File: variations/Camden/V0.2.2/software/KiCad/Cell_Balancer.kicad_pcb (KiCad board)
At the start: 2 copper layers, 14 parts, among them J1 Screw_Terminal_01x11, J2 DC37_Pins

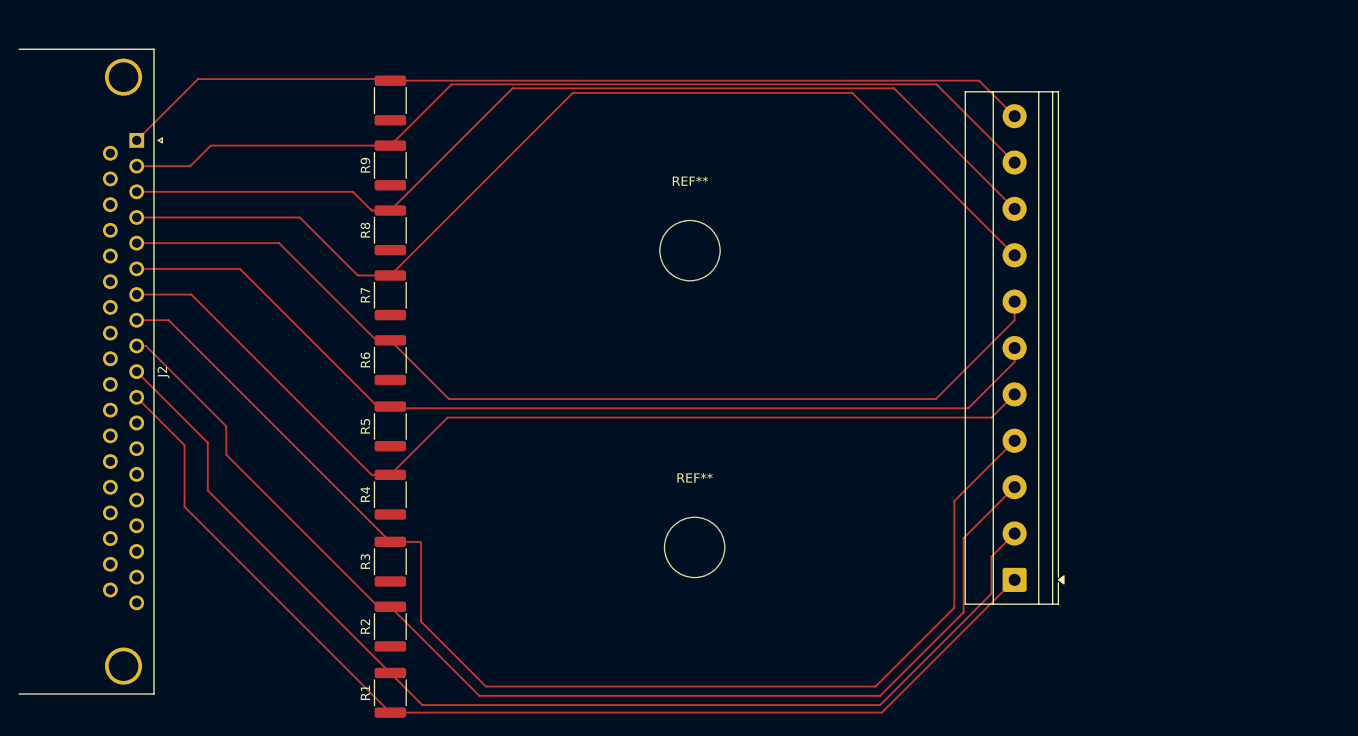
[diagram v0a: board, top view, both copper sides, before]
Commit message: update
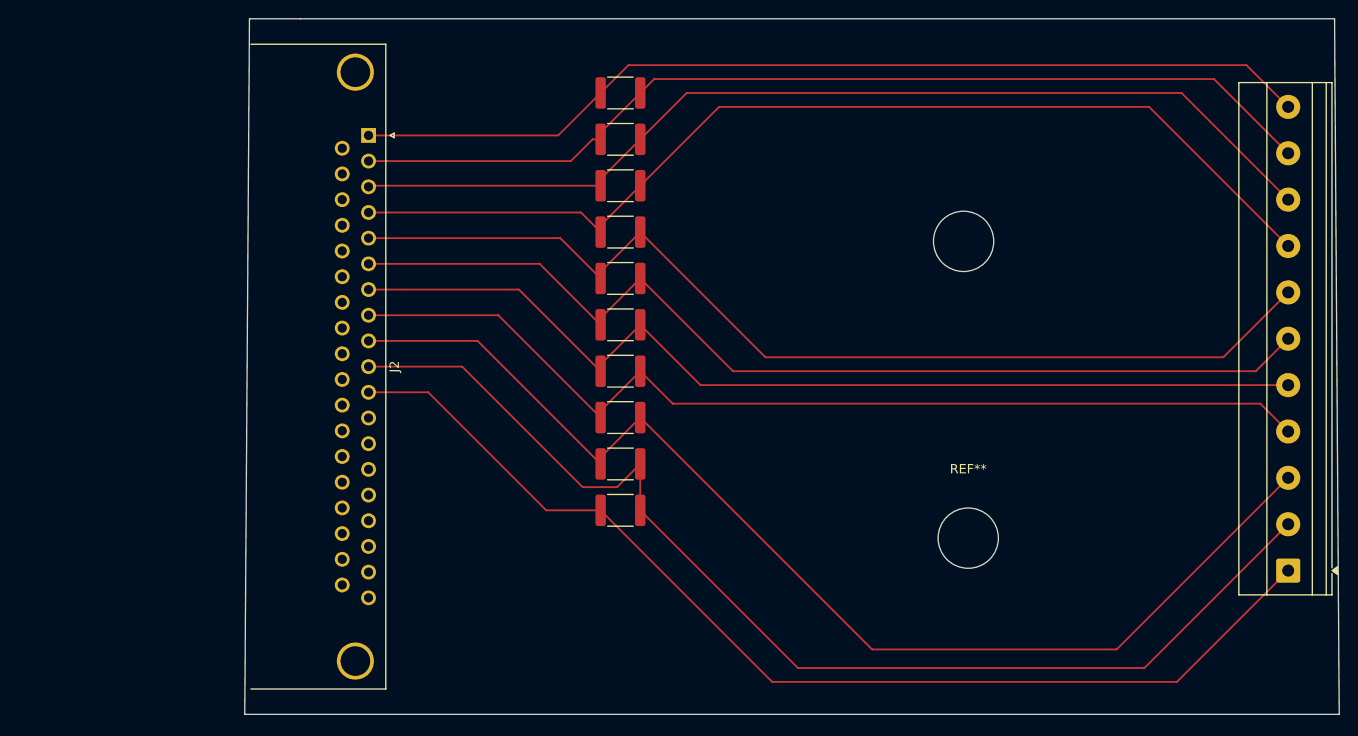
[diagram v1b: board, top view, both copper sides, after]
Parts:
- moved R1 31.7 mm to (124.5, 128.0), turned to 0 degrees
- moved R2 30.4 mm to (124.5, 123.0), turned to 180 degrees
- moved J1 29.5 mm to (196.5, 134.5)
- moved REF** 29.5 mm to (161.5, 99.0)
- moved REF** 29.5 mm to (162.0, 131.0)
- moved R3 29.3 mm to (124.5, 118.0), turned to 180 degrees
- moved R4 28.2 mm to (124.5, 113.0), turned to 180 degrees
- moved R5 27.1 mm to (124.5, 108.0), turned to 180 degrees
- moved R6 26.3 mm to (124.5, 103.0), turned to 180 degrees
- moved R7 25.7 mm to (124.5, 98.0), turned to 180 degrees
- moved R8 25.3 mm to (124.5, 93.0), turned to 180 degrees
- moved J2 25.0 mm to (97.3, 87.6)
- moved R9 25.0 mm to (124.5, 88.0), turned to 180 degrees
- moved R10 24.8 mm to (124.5, 83.0), turned to 180 degrees
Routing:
- net Net-(J1-Pin_4): track 133.7 -> 108.9 mm
- net Net-(J1-Pin_6): track 104.5 -> 110.0 mm
- net Net-(J1-Pin_11): track 99.1 -> 104.2 mm
- net Net-(J1-Pin_7): track 107.1 -> 111.9 mm
- net Net-(J1-Pin_10): track 101.8 -> 106.6 mm
- net Net-(J1-Pin_9): track 106.3 -> 108.5 mm
- net Net-(J1-Pin_5): track 106.3 -> 108.0 mm
- net Net-(J1-Pin_1): track 118.6 -> 117.1 mm
- net Net-(J1-Pin_2): track 122.6 -> 124.0 mm
- net Net-(J1-Pin_3): track 126.1 -> 125.2 mm
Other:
- board outline added: 118 x 75 mm

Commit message: update
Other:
- board text added: "Cebastione Bailey Cell Balancer V.2.20 ARTS-Lab 9-1-2026"
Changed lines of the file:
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@@
 		(layer "Edge.Cuts")
+	)
+	(gr_text "Cebastione Bailey\nCell Balancer V.2.20\nARTS-Lab\n9-1-2026\n"
+		(at 100.5 136.5 0)
+		(layer "Edge.Cuts")
+		(effects
+			(font
+				(size 1 1)
+				(thickness 0.15)
+			)
+			(justify left bottom)
+		)
 	)
 	(segment
